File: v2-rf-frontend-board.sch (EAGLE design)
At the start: 153 parts, among them J3 ROCKETNET-CONNECTOR-16M, Q1 NTR4101P, T1 ALT4532, T2 ALT4532, U1 MAX2769, U10 LMZ12001, U2 SAW, U3 LAN8710A-EZC, U4 7Q-16.368MBG-T, U5 XC2401, U6 MAX8510EXK29+T, U7 MAX8510EXK29+T, U8 STM32F4V, X1 25 MHz, X2 BU-SMA-H

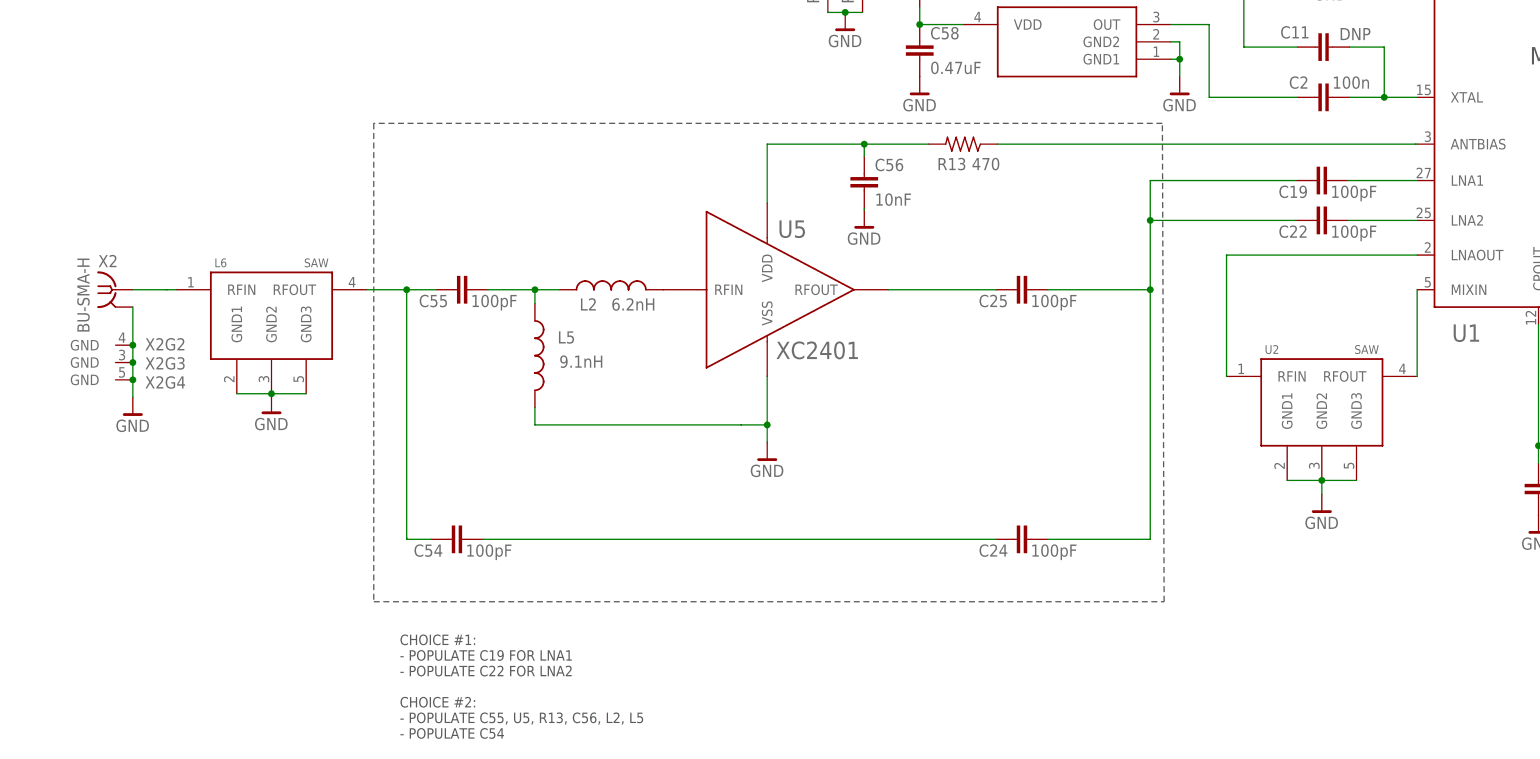
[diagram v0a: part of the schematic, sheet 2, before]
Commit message: Made a capacitor options footprint and symbol for the 'do not populate' choice capacitor hack.
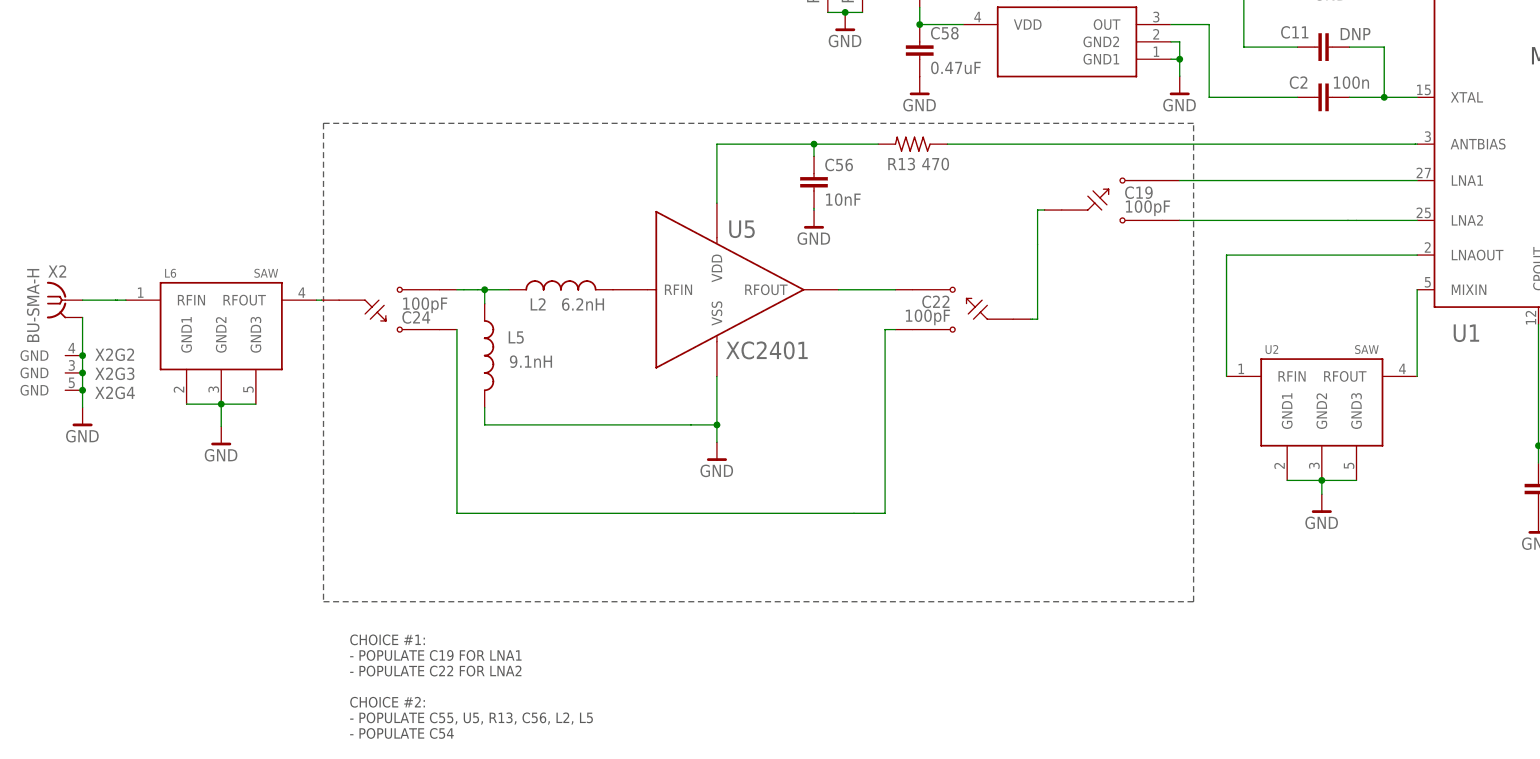
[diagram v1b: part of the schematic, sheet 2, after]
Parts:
- removed C25, C54, C55: 100pF, rcl:C-EUC0402
- C19, C22, C24: device rcl:C-EUC0402 -> wicker:CAP-OPTION
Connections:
- removed net N$1: C22.2, U1.LNA2
- new net N$25: C19.2, C22.2
- net N$17: now also C19.3, U1.LNA2; no longer C19.1, C22.1, C24.2, C25.2
- net N$2: now also C19.1; no longer C19.2
- net N$21: now also C24.2; no longer C54.1, C55.1
- net N$22: now also C24.3; no longer C55.2
- net N$3: now also C22.1; no longer C25.1
- net N$5: now also C22.3; no longer C54.2
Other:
- moved on the sheet: C56, L2, L5, L6, R13, U5, X2, X2G2, X2G3, X2G4

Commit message: Laid out new LNA1, LNA2, and ANTBIAS sections. Layout done. Passes ERC, DRC. Ready for design review.
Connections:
- net N$23 renamed ANTBIAS
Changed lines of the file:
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@@
 </segment>
 </net>
-<net name="N$23" class="0">
+<net name="ANTBIAS" class="0">
 <segment>
 <pinref part="R13" gate="G$1" pin="1"/>
